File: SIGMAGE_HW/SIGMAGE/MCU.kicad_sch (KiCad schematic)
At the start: 51 parts, among them J5 TSW10607GS, U15 STM32F407VGTx, X1 STDCSU18M

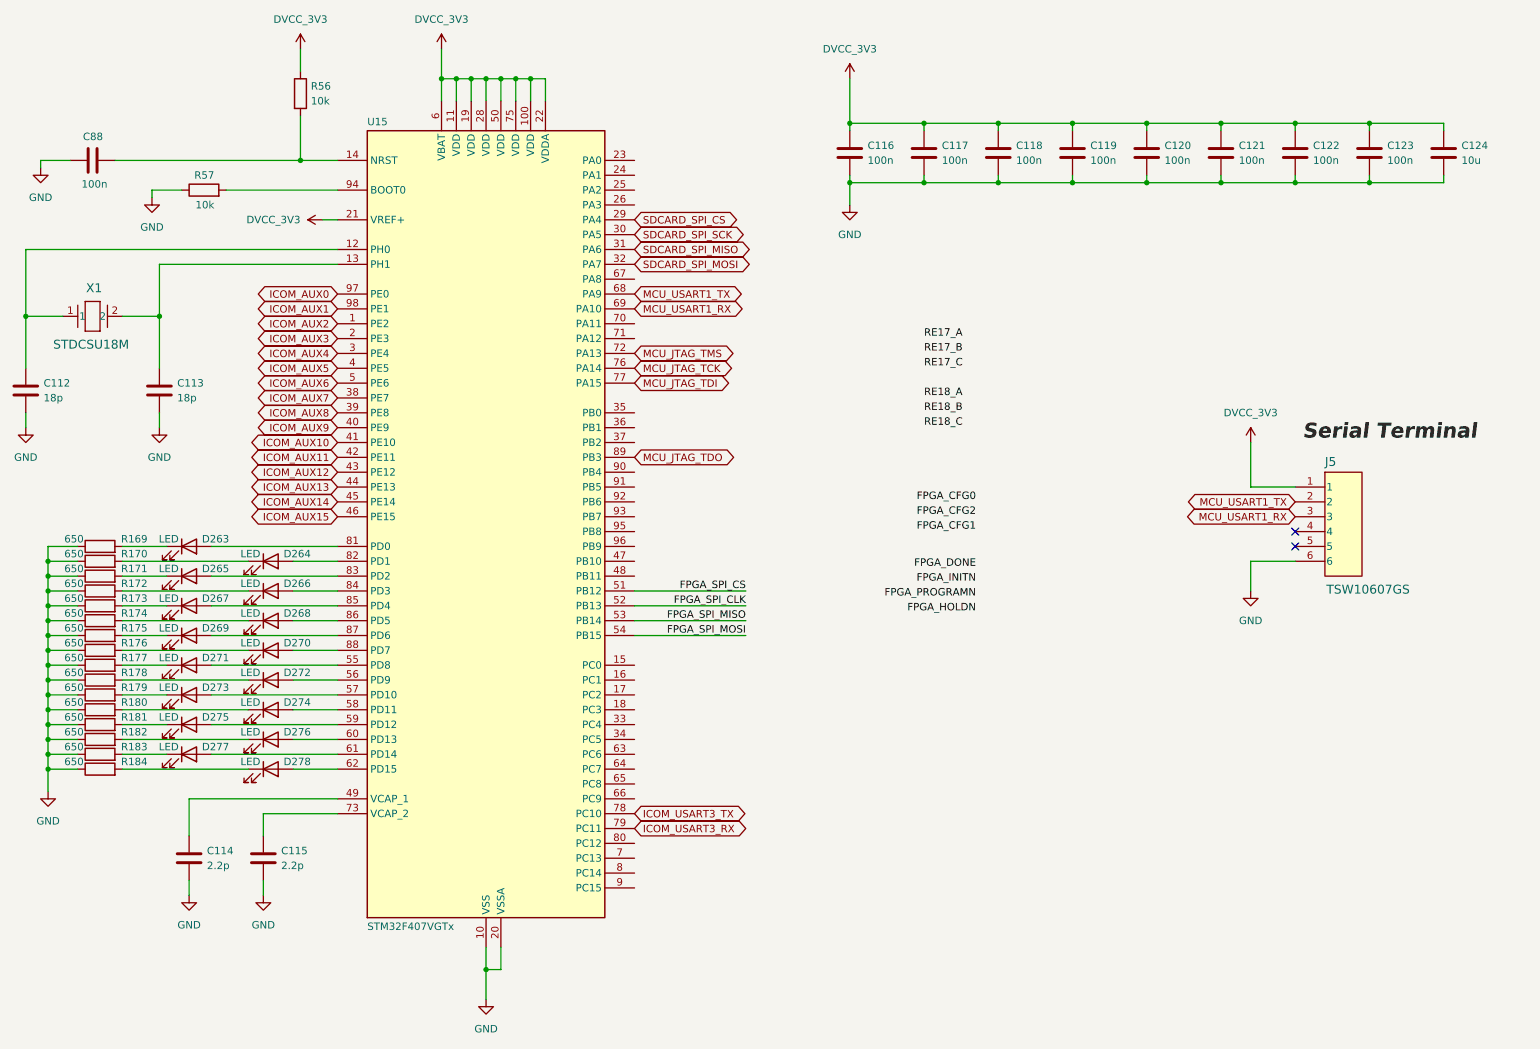
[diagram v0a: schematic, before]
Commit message: finished schematic
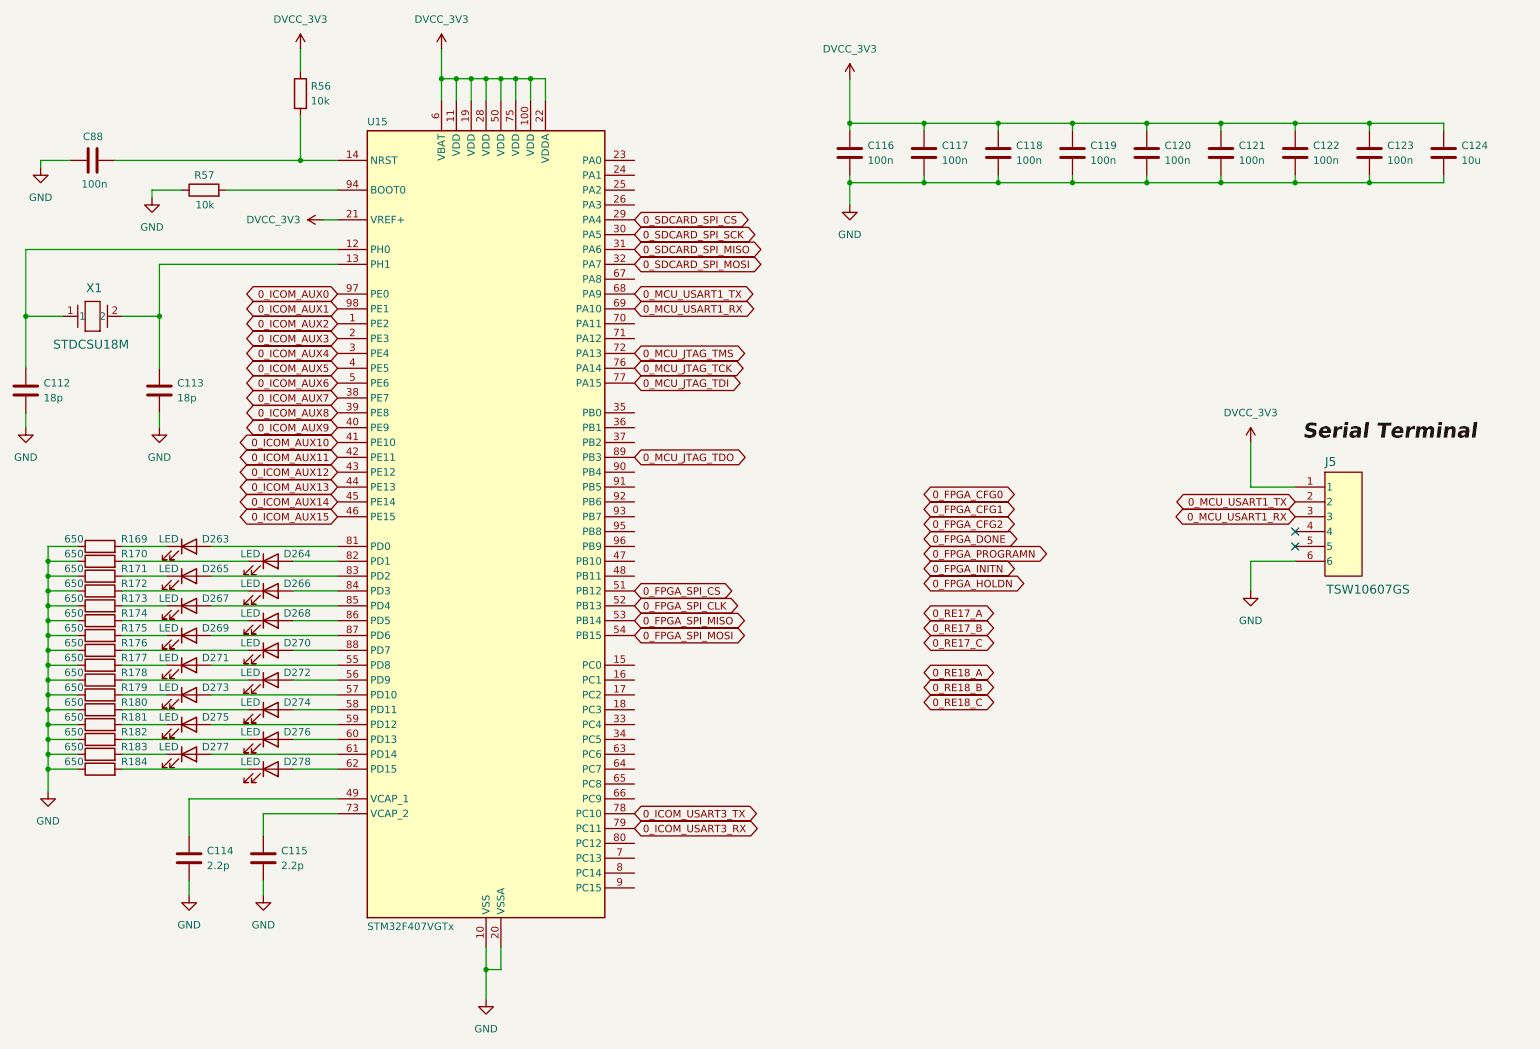
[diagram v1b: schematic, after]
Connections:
- net FPGA_SPI_CLK renamed 0_FPGA_SPI_CLK
- net FPGA_SPI_CS renamed 0_FPGA_SPI_CS
- net FPGA_SPI_MISO renamed 0_FPGA_SPI_MISO
- net FPGA_SPI_MOSI renamed 0_FPGA_SPI_MOSI
- net ICOM_AUX0 renamed 0_ICOM_AUX0
- net ICOM_AUX1 renamed 0_ICOM_AUX1
- net ICOM_AUX10 renamed 0_ICOM_AUX10
- net ICOM_AUX11 renamed 0_ICOM_AUX11
- net ICOM_AUX12 renamed 0_ICOM_AUX12
- net ICOM_AUX13 renamed 0_ICOM_AUX13
- net ICOM_AUX14 renamed 0_ICOM_AUX14
- net ICOM_AUX15 renamed 0_ICOM_AUX15
- net ICOM_AUX2 renamed 0_ICOM_AUX2
- net ICOM_AUX3 renamed 0_ICOM_AUX3
- net ICOM_AUX4 renamed 0_ICOM_AUX4
- net ICOM_AUX5 renamed 0_ICOM_AUX5
- net ICOM_AUX6 renamed 0_ICOM_AUX6
- net ICOM_AUX7 renamed 0_ICOM_AUX7
- net ICOM_AUX8 renamed 0_ICOM_AUX8
- net ICOM_AUX9 renamed 0_ICOM_AUX9
- net ICOM_USART3_RX renamed 0_ICOM_USART3_RX
- net ICOM_USART3_TX renamed 0_ICOM_USART3_TX
- net MCU_JTAG_TCK renamed 0_MCU_JTAG_TCK
- net MCU_JTAG_TDI renamed 0_MCU_JTAG_TDI
- net MCU_JTAG_TDO renamed 0_MCU_JTAG_TDO
- net MCU_JTAG_TMS renamed 0_MCU_JTAG_TMS
- net MCU_USART1_RX renamed 0_MCU_USART1_RX
- net MCU_USART1_TX renamed 0_MCU_USART1_TX
- net SDCARD_SPI_CS renamed 0_SDCARD_SPI_CS
- net SDCARD_SPI_MISO renamed 0_SDCARD_SPI_MISO
- net SDCARD_SPI_MOSI renamed 0_SDCARD_SPI_MOSI
- net SDCARD_SPI_SCK renamed 0_SDCARD_SPI_SCK

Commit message: basic layout
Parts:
- C88: footprint Capacitor_SMD:C_1206_3216Metric -> Capacitor_SMD:C_0603_1608Metric
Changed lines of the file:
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@@
 			)
 		)
-		(property "Footprint" "Capacitor_SMD:C_1206_3216Metric"
+		(property "Footprint" "Capacitor_SMD:C_0603_1608Metric"
 			(at 40.64 42.2148 0)
 			(hide yes)

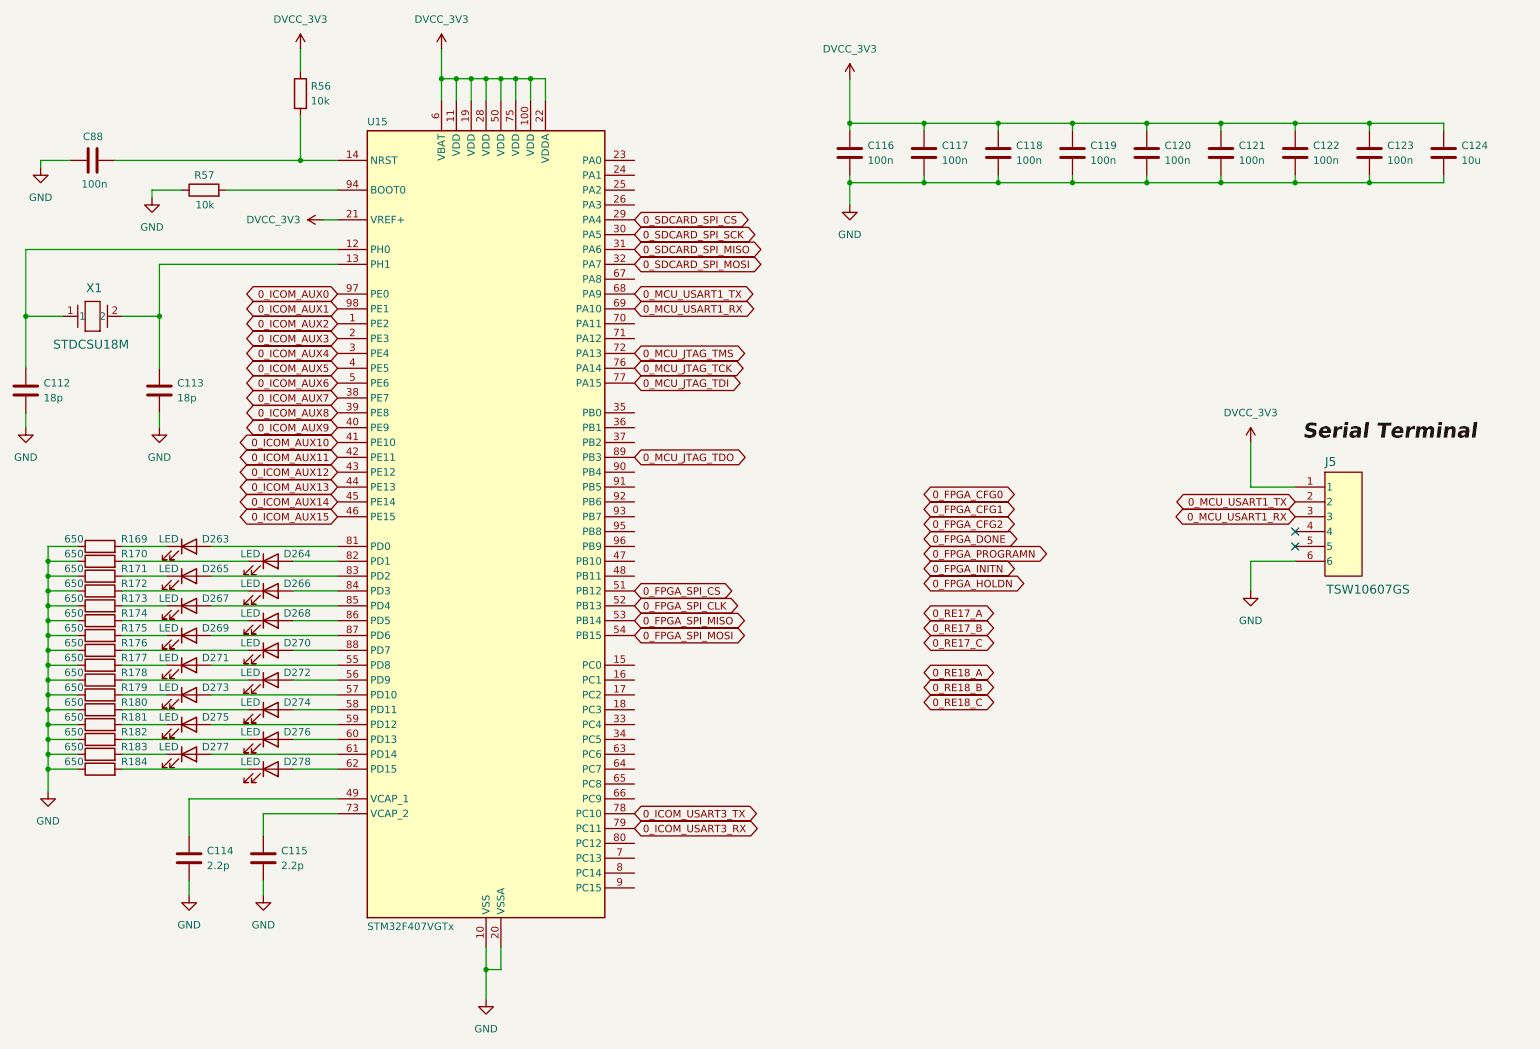
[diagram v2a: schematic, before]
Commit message: uga uga
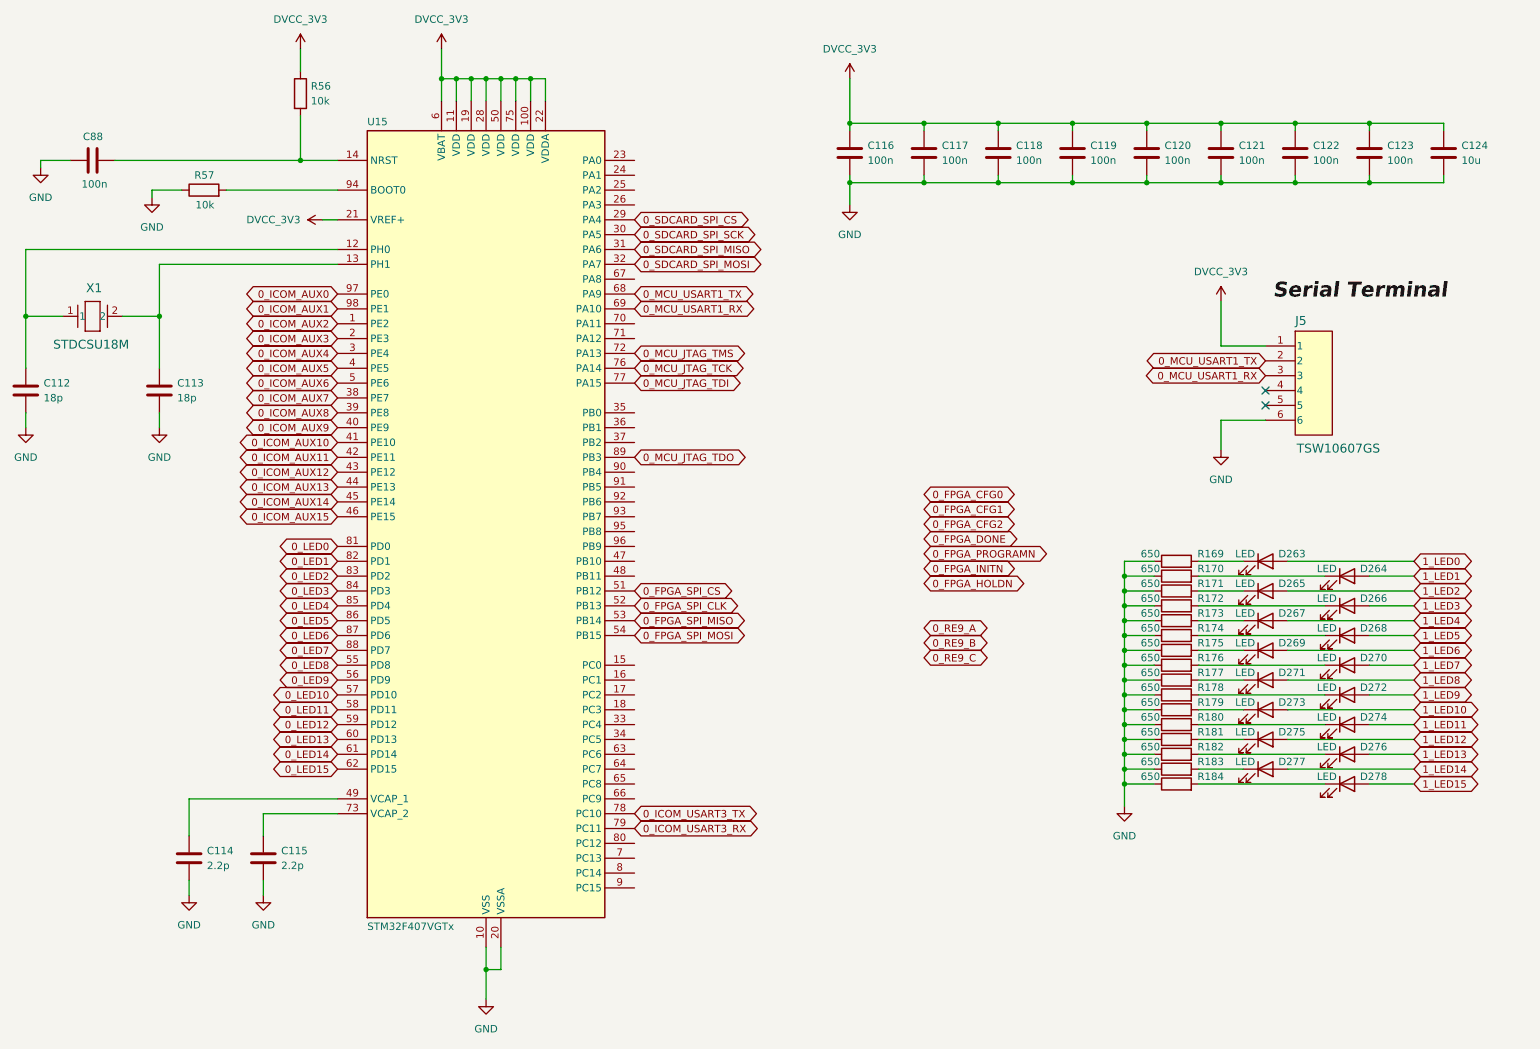
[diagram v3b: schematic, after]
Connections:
- net 0_LED0: now reaches U15.81 (PD0)
- net 0_LED0: no longer D263.2 (A)
- net 0_LED10: now reaches U15.57 (PD10)
- net 0_LED10: no longer D273.2 (A)
- net 0_LED12: now reaches U15.59 (PD12)
- net 0_LED12: no longer D275.2 (A)
- net 0_LED2: now reaches U15.83 (PD2)
- net 0_LED2: no longer D265.2 (A)
- net 0_LED3: now reaches U15.84 (PD3)
- net 0_LED3: no longer D266.2 (A)
- net 0_LED8: now reaches U15.55 (PD8)
- net 0_LED8: no longer D271.2 (A)
- net 0_LED9: now reaches U15.56 (PD9)
- net 0_LED9: no longer D272.2 (A)
- net 0_LED11: now reaches U15.58 (PD11)
- net 0_LED11: no longer D274.2 (A)
- net 0_LED13: now reaches U15.60 (PD13)
- net 0_LED13: no longer D276.2 (A)
- net 0_LED14: now reaches U15.61 (PD14)
- net 0_LED14: no longer D277.2 (A)
- net 0_LED15: now reaches U15.62 (PD15)
- net 0_LED15: no longer D278.2 (A)
- net 0_LED1: now reaches U15.82 (PD1)
- net 0_LED1: no longer D264.2 (A)
- net 0_LED4: now reaches U15.85 (PD4)
- net 0_LED4: no longer D267.2 (A)
- net 0_LED5: now reaches U15.86 (PD5)
- net 0_LED5: no longer D268.2 (A)
- net 0_LED6: now reaches U15.87 (PD6)
- net 0_LED6: no longer D269.2 (A)
- net 0_LED7: now reaches U15.88 (PD7)
- net 0_LED7: no longer D270.2 (A)
- new net 1_LED0: D263.2 (A)
- new net 1_LED1: D264.2 (A)
- new net 1_LED10: D273.2 (A)
- new net 1_LED11: D274.2 (A)
- new net 1_LED12: D275.2 (A)
- new net 1_LED13: D276.2 (A)
- new net 1_LED14: D277.2 (A)
- new net 1_LED15: D278.2 (A)
- new net 1_LED2: D265.2 (A)
- new net 1_LED3: D266.2 (A)
- new net 1_LED4: D267.2 (A)
- new net 1_LED5: D268.2 (A)
- new net 1_LED6: D269.2 (A)
- new net 1_LED7: D270.2 (A)
- new net 1_LED8: D271.2 (A)
- new net 1_LED9: D272.2 (A)
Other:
- moved on the sheet: J5

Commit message: more routing
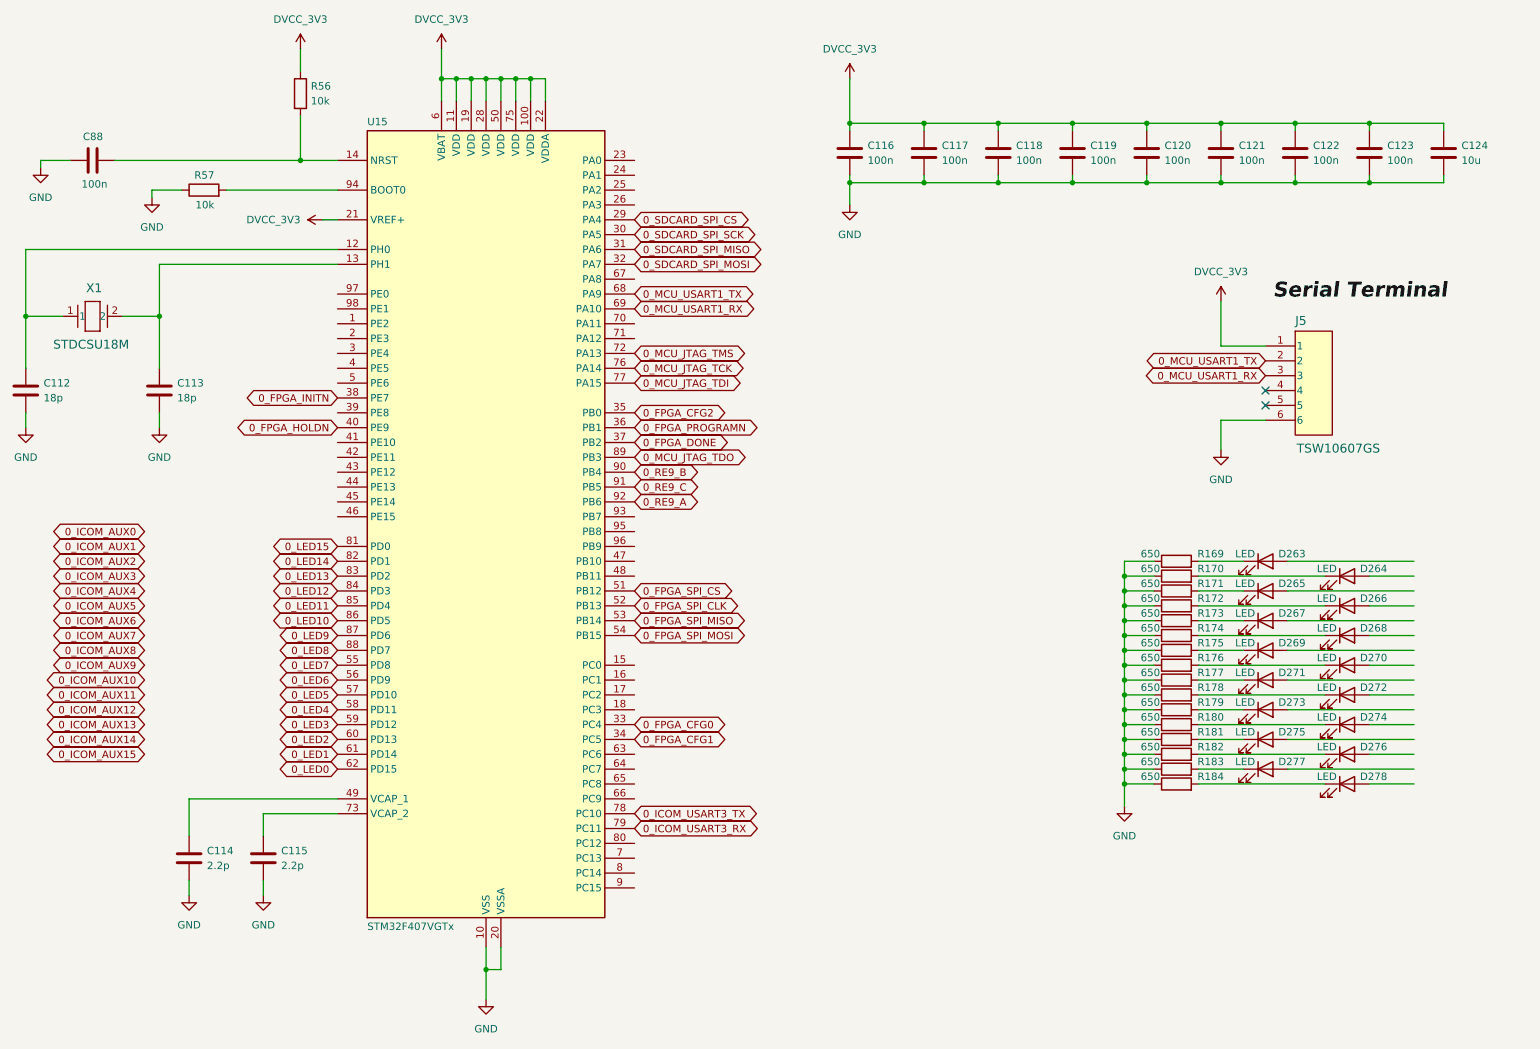
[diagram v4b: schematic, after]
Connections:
- net 0_FPGA_CFG0: now also U15.33 (PC4)
- net 0_FPGA_CFG1: now also U15.34 (PC5)
- net 0_FPGA_CFG2: now also U15.35 (PB0)
- net 0_FPGA_DONE: now also U15.37 (PB2)
- net 0_FPGA_HOLDN: now also U15.40 (PE9)
- net 0_FPGA_INITN: now also U15.38 (PE7)
- net 0_FPGA_PROGRAMN: now also U15.36 (PB1)
- net 0_ICOM_AUX0: no longer U15.97 (PE0)
- net 0_ICOM_AUX1: no longer U15.98 (PE1)
- net 0_ICOM_AUX10: no longer U15.41 (PE10)
- net 0_ICOM_AUX11: no longer U15.42 (PE11)
- net 0_ICOM_AUX12: no longer U15.43 (PE12)
- net 0_ICOM_AUX13: no longer U15.44 (PE13)
- net 0_ICOM_AUX14: no longer U15.45 (PE14)
- net 0_ICOM_AUX15: no longer U15.46 (PE15)
- net 0_ICOM_AUX2: no longer U15.1 (PE2)
- net 0_ICOM_AUX3: no longer U15.2 (PE3)
- net 0_ICOM_AUX4: no longer U15.3 (PE4)
- net 0_ICOM_AUX5: no longer U15.4 (PE5)
- net 0_ICOM_AUX6: no longer U15.5 (PE6)
- net 0_ICOM_AUX7: no longer U15.38 (PE7)
- net 0_ICOM_AUX8: no longer U15.39 (PE8)
- net 0_ICOM_AUX9: no longer U15.40 (PE9)
- net 0_LED0: now also U15.62 (PD15); no longer U15.81 (PD0)
- net 0_LED1: now also U15.61 (PD14); no longer U15.82 (PD1)
- net 0_LED10: now also U15.86 (PD5); no longer U15.57 (PD10)
- net 0_LED11: now also U15.85 (PD4); no longer U15.58 (PD11)
- net 0_LED12: now also U15.84 (PD3); no longer U15.59 (PD12)
- net 0_LED13: now also U15.83 (PD2); no longer U15.60 (PD13)
- net 0_LED14: now also U15.82 (PD1); no longer U15.61 (PD14)
- net 0_LED15: now also U15.81 (PD0); no longer U15.62 (PD15)
- net 0_LED2: now also U15.60 (PD13); no longer U15.83 (PD2)
- net 0_LED3: now also U15.59 (PD12); no longer U15.84 (PD3)
- net 0_LED4: now also U15.58 (PD11); no longer U15.85 (PD4)
- net 0_LED5: now also U15.57 (PD10); no longer U15.86 (PD5)
- net 0_LED6: now also U15.56 (PD9); no longer U15.87 (PD6)
- net 0_LED7: now also U15.55 (PD8); no longer U15.88 (PD7)
- net 0_LED8: now also U15.88 (PD7); no longer U15.55 (PD8)
- net 0_LED9: now also U15.87 (PD6); no longer U15.56 (PD9)
- net 0_RE9_A: now also U15.92 (PB6)
- net 0_RE9_B: now also U15.90 (PB4)
- net 0_RE9_C: now also U15.91 (PB5)
- net 1_LED0: no longer names the net of D263.2 (A)
- net 1_LED1: no longer names the net of D264.2 (A)
- net 1_LED10: no longer names the net of D273.2 (A)
- net 1_LED11: no longer names the net of D274.2 (A)
- net 1_LED12: no longer names the net of D275.2 (A)
- net 1_LED13: no longer names the net of D276.2 (A)
- net 1_LED14: no longer names the net of D277.2 (A)
- net 1_LED15: no longer names the net of D278.2 (A)
- net 1_LED2: no longer names the net of D265.2 (A)
- net 1_LED3: no longer names the net of D266.2 (A)
- net 1_LED4: no longer names the net of D267.2 (A)
- net 1_LED5: no longer names the net of D268.2 (A)
- net 1_LED6: no longer names the net of D269.2 (A)
- net 1_LED7: no longer names the net of D270.2 (A)
- net 1_LED8: no longer names the net of D271.2 (A)
- net 1_LED9: no longer names the net of D272.2 (A)
